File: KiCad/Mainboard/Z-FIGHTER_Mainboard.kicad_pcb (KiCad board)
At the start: 2 copper layers, 100 x 150 mm, 52 parts, among them IC1 Z80SIO, J1 DB9_Male_MountingHoles, J2 DB9_Male_MountingHoles, J3 USB_B, J4 Conn_02x13_Odd_Even, J5 Conn_Parallel_User, J6 Conn_PATA, J7 Conn_02x03_Odd_Even, SW1 SW_Push, SW2 SW_DIP_x03, U1 AS6C4008-55PCN, U10 DS1233, U2 Z80CPU, U3 82C55A, U4 SST39SF040, U5 MAX203, U6 MAX203, U7 ATF22V10CZ-15PI, U8 74HC00, U9 82C55A, X1 Z80/SIO Ch.A Clock, X2 SIO Ch.B Clock

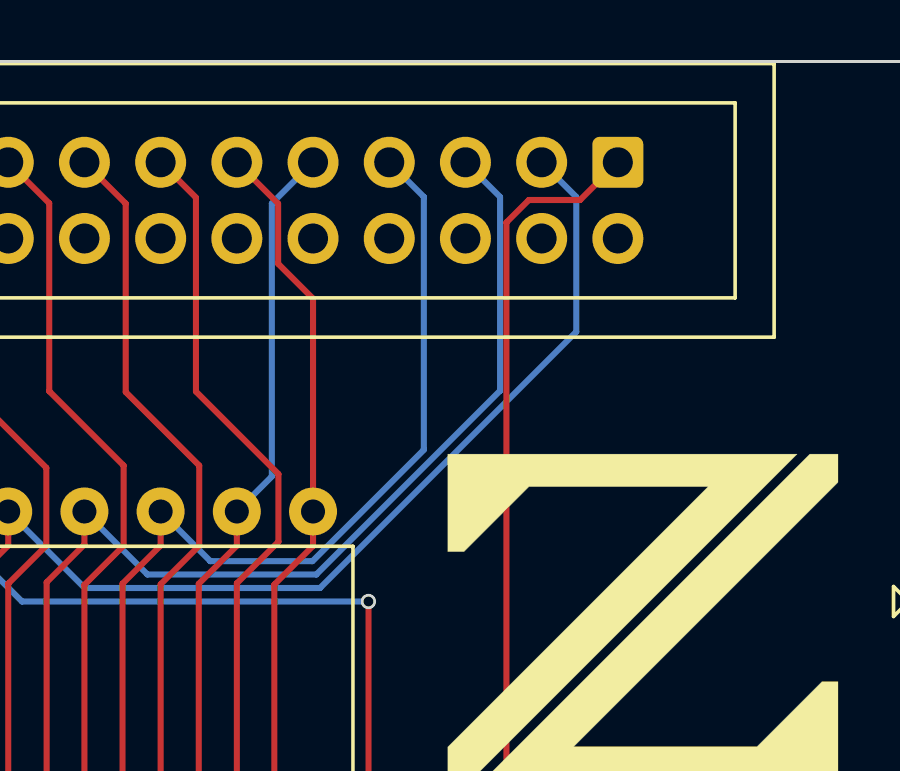
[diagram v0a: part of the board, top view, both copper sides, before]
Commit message: Update Z-FIGHTER_Mainboard.kicad_pcb
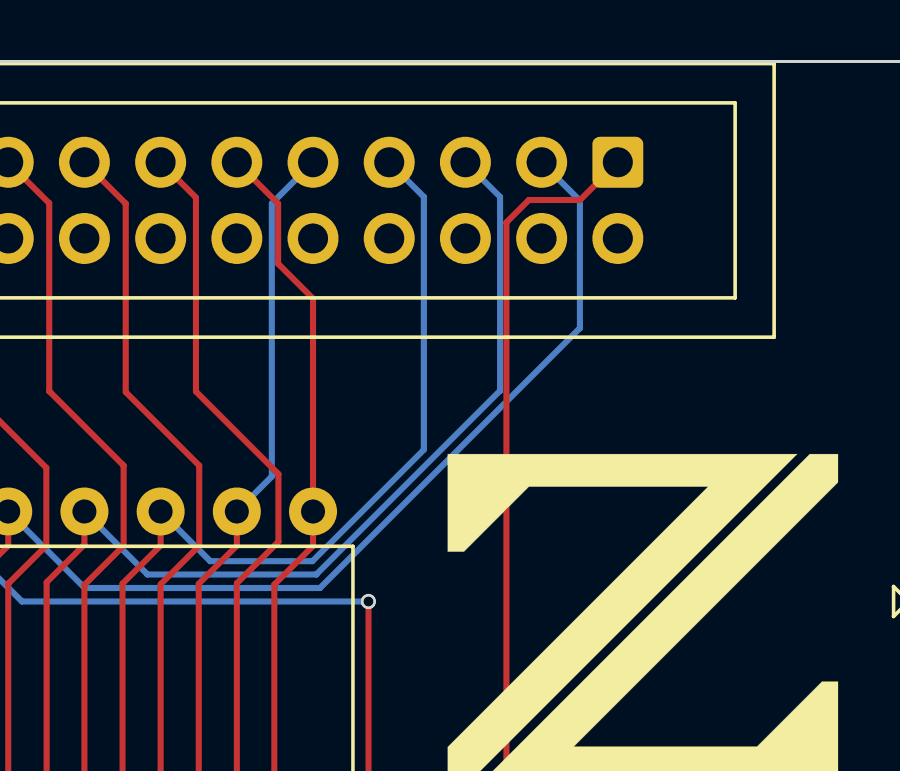
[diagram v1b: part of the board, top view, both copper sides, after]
